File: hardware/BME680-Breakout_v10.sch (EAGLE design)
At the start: 23 parts, among them IC1 BME680, IC2 LDO-TS9011-3V3, J1 JUMPER2-0603, T1 BSS138PS, T2 BSS138PS, X1 PASSER-07, X2 PASSER-07

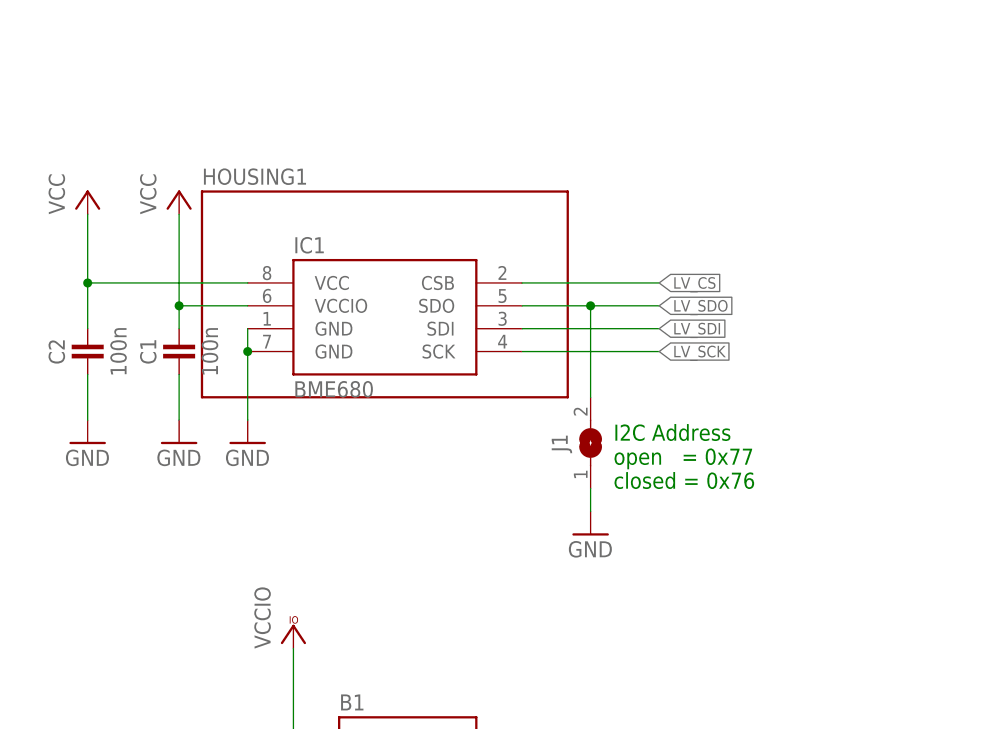
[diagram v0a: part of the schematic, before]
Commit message: updated layout and schematic
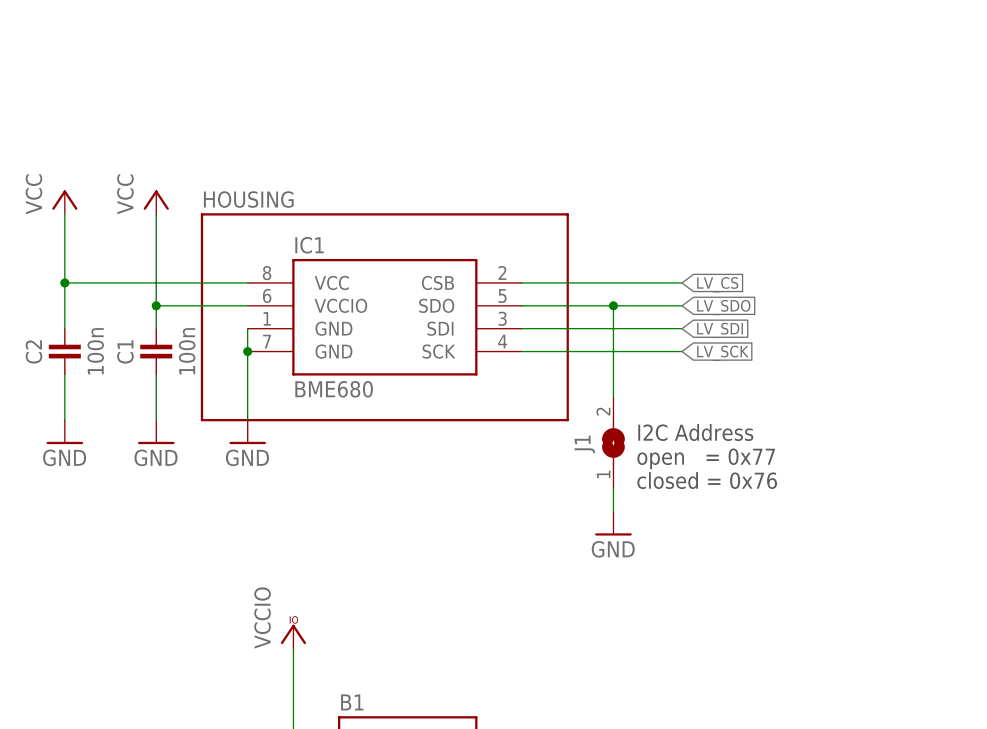
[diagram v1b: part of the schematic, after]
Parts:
- removed HOUSING1: SF2, we-sensor:SF2
- added HOUSING: SF2, we-sensor:SF2
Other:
- moved on the sheet: C1, C2, J1
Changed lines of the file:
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@@
 <setting verticaltext="up"/>
 </settings>
-<grid distance="0.1" unitdist="inch" unit="inch" style="lines" multiple="1" display="no" altdistance="0.01" altunitdist="inch" altunit="inch"/>
+<grid distance="0.05" unitdist="inch" unit="inch" style="lines" multiple="1" display="yes" altdistance="0.025" altunitdist="inch" altunit="inch"/>
 <layers>
 <layer number="1" name="Top" color="4" fill="1" visible="no" active="no"/>
@@
 <part name="J1" library="we-rcl" deviceset="JUMPER2" device="-0603"/>
 <part name="GND8" library="supply1" deviceset="GND" device=""/>
-<part name="HOUSING1" library="we-sensor" deviceset="SF2" device=""/>
+<part name="HOUSING" library="we-sensor" deviceset="SF2" device=""/>
 <part name="IC1" library="we-sensor" deviceset="BME680" device=""/>
 </parts>
@@
 <sheet>
 <plain>
-<text x="109.22" y="119.38" size="1.778" layer="91">I2C Address
+<text x="111.76" y="119.38" size="1.778" layer="97">I2C Address
 open   = 0x77
 closed = 0x76</text>
@@
 <instances>
 <instance part="B1" gate="BOARD" x="86.36" y="83.82"/>
-<instance part="GND1" gate="1" x="60.96" y="124.46"/>
-<instance part="P+1" gate="VCC" x="50.8" y="152.4"/>
-<instance part="C1" gate="C" x="60.96" y="134.62" rot="R90"/>
+<instance part="GND1" gate="1" x="58.42" y="124.46"/>
+<instance part="P+1" gate="VCC" x="48.26" y="152.4"/>
+<instance part="C1" gate="C" x="58.42" y="134.62" rot="R90"/>
 <instance part="R1" gate="R" x="191.77" y="154.94" rot="R90"/>
 <instance part="IC2" gate="A" x="86.36" y="43.18"/>
@@
 <attribute name="VALUE" x="201.93" y="33.02" size="1.778" layer="96"/>
 </instance>
-<instance part="P+2" gate="VCC" x="60.96" y="152.4"/>
-<instance part="C2" gate="C" x="50.8" y="134.62" rot="R90"/>
+<instance part="P+2" gate="VCC" x="58.42" y="152.4"/>
+<instance part="C2" gate="C" x="48.26" y="134.62" rot="R90"/>
 <instance part="GND2" gate="1" x="68.58" y="124.46"/>
-<instance part="GND3" gate="1" x="50.8" y="124.46"/>
+<instance part="GND3" gate="1" x="48.26" y="124.46"/>
 <instance part="R2" gate="R" x="217.17" y="154.94" rot="R90"/>
 <instance part="R3" gate="R" x="191.77" y="119.38" rot="R90"/>
@@
 <instance part="LOGO1" gate="L" x="207.01" y="7.62"/>
 <instance part="LOGO2" gate="L" x="194.31" y="7.62"/>
-<instance part="J1" gate="J" x="106.68" y="124.46" rot="R90"/>
-<instance part="GND8" gate="1" x="106.68" y="114.3"/>
-<instance part="HOUSING1" gate="G$1" x="83.82" y="139.7"/>
-<instance part="IC1" gate="G$1" x="83.82" y="137.16"/>
+<instance part="J1" gate="J" x="109.22" y="124.46" rot="R90"/>
+<instance part="GND8" gate="1" x="109.22" y="114.3"/>
+<instance part="HOUSING" gate="G$1" x="83.82" y="137.16"/>
+<instance part="IC1" gate="IC" x="83.82" y="137.16"/>
 </instances>
 <busses>
@@
 <segment>
 <pinref part="P+1" gate="VCC" pin="VCC"/>
-<wire x1="68.58" y1="142.24" x2="50.8" y2="142.24" width="0.1524" layer="91"/>
-<wire x1="50.8" y1="142.24" x2="50.8" y2="149.86" width="0.1524" layer="91"/>
+<wire x1="68.58" y1="142.24" x2="48.26" y2="142.24" width="0.1524" layer="91"/>
+<wire x1="48.26" y1="142.24" x2="48.26" y2="149.86" width="0.1524" layer="91"/>
 <pinref part="C2" gate="C" pin="2"/>
-<wire x1="50.8" y1="137.16" x2="50.8" y2="142.24" width="0.1524" layer="91"/>
-<junction x="50.8" y="142.24"/>
-<pinref part="IC1" gate="G$1" pin="VCC"/>
+<wire x1="48.26" y1="137.16" x2="48.26" y2="142.24" width="0.1524" layer="91"/>
+<junction x="48.26" y="142.24"/>
+<pinref part="IC1" gate="IC" pin="VCC"/>
 </segment>
 <segment>
 <pinref part="P+2" gate="VCC" pin="VCC"/>
-<wire x1="68.58" y1="139.7" x2="60.96" y2="139.7" width="0.1524" layer="91"/>
-<wire x1="60.96" y1="139.7" x2="60.96" y2="149.86" width="0.1524" layer="91"/>
+<wire x1="68.58" y1="139.7" x2="58.42" y2="139.7" width="0.1524" layer="91"/>
+<wire x1="58.42" y1="139.7" x2="58.42" y2="149.86" width="0.1524" layer="91"/>
 <pinref part="C1" gate="C" pin="2"/>
-<wire x1="60.96" y1="137.16" x2="60.96" y2="139.7" width="0.1524" layer="91"/>
-<junction x="60.96" y="139.7"/>
-<pinref part="IC1" gate="G$1" pin="VCCIO"/>
+<wire x1="58.42" y1="137.16" x2="58.42" y2="139.7" width="0.1524" layer="91"/>
+<junction x="58.42" y="139.7"/>
+<pinref part="IC1" gate="IC" pin="VCCIO"/>
 </segment>
 <segment>
@@
 <wire x1="68.58" y1="134.62" x2="68.58" y2="127" width="0.1524" layer="91"/>
 <junction x="68.58" y="134.62"/>
-<pinref part="IC1" gate="G$1" pin="GND@1"/>
-<pinref part="IC1" gate="G$1" pin="GND@2"/>
+<pinref part="IC1" gate="IC" pin="GND@1"/>
+<pinref part="IC1" gate="IC" pin="GND@2"/>
 </segment>
 <segment>
 <pinref part="GND3" gate="1" pin="GND"/>
 <pinref part="C2" gate="C" pin="1"/>
-<wire x1="50.8" y1="127" x2="50.8" y2="132.08" width="0.1524" layer="91"/>
+<wire x1="48.26" y1="127" x2="48.26" y2="132.08" width="0.1524" layer="91"/>
 </segment>
 <segment>
 <pinref part="C1" gate="C" pin="1"/>
 <pinref part="GND1" gate="1" pin="GND"/>
-<wire x1="60.96" y1="132.08" x2="60.96" y2="127" width="0.1524" layer="91"/>
+<wire x1="58.42" y1="132.08" x2="58.42" y2="127" width="0.1524" layer="91"/>
 </segment>
 <segment>
@@
 <pinref part="GND8" gate="1" pin="GND"/>
 <pinref part="J1" gate="J" pin="1"/>
-<wire x1="106.68" y1="116.84" x2="106.68" y2="119.38" width="0.1524" layer="91"/>
+<wire x1="109.22" y1="116.84" x2="109.22" y2="119.38" width="0.1524" layer="91"/>
 </segment>
 </net>
 <net name="LV_SDO" class="0">
 <segment>
-<wire x1="99.06" y1="139.7" x2="106.68" y2="139.7" width="0.1524" layer="91"/>
-<label x="114.3" y="139.7" size="1.27" layer="95" xref="yes"/>
+<wire x1="99.06" y1="139.7" x2="109.22" y2="139.7" width="0.1524" layer="91"/>
+<label x="116.84" y="139.7" size="1.27" layer="95" xref="yes"/>
 <pinref part="J1" gate="J" pin="2"/>
-<wire x1="106.68" y1="139.7" x2="114.3" y2="139.7" width="0.1524" layer="91"/>
-<wire x1="106.68" y1="129.54" x2="106.68" y2="139.7" width="0.1524" layer="91"/>
-<junction x="106.68" y="139.7"/>
-<pinref part="IC1" gate="G$1" pin="SDO"/>
+<wire x1="109.22" y1="139.7" x2="116.84" y2="139.7" width="0.1524" layer="91"/>
+<wire x1="109.22" y1="129.54" x2="109.22" y2="139.7" width="0.1524" layer="91"/>
+<junction x="109.22" y="139.7"/>
+<pinref part="IC1" gate="IC" pin="SDO"/>
 </segment>
 <segment>
@@
 <net name="LV_CS" class="0">
 <segment>
-<wire x1="99.06" y1="142.24" x2="114.3" y2="142.24" width="0.1524" layer="91"/>
-<label x="114.3" y="142.24" size="1.27" layer="95" xref="yes"/>
-<pinref part="IC1" gate="G$1" pin="CSB"/>
+<wire x1="99.06" y1="142.24" x2="116.84" y2="142.24" width="0.1524" layer="91"/>
+<label x="116.84" y="142.24" size="1.27" layer="95" xref="yes"/>
+<pinref part="IC1" gate="IC" pin="CSB"/>
 </segment>
 <segment>
@@
 <net name="LV_SDI" class="0">
 <segment>
-<wire x1="99.06" y1="137.16" x2="114.3" y2="137.16" width="0.1524" layer="91"/>
-<label x="114.3" y="137.16" size="1.27" layer="95" xref="yes"/>
-<pinref part="IC1" gate="G$1" pin="SDI"/>
+<wire x1="99.06" y1="137.16" x2="116.84" y2="137.16" width="0.1524" layer="91"/>
+<label x="116.84" y="137.16" size="1.27" layer="95" xref="yes"/>
+<pinref part="IC1" gate="IC" pin="SDI"/>
 </segment>
 <segment>
@@
 <net name="LV_SCK" class="0">
 <segment>
-<wire x1="99.06" y1="134.62" x2="114.3" y2="134.62" width="0.1524" layer="91"/>
-<label x="114.3" y="134.62" size="1.27" layer="95" xref="yes"/>
-<pinref part="IC1" gate="G$1" pin="SCK"/>
-</segment>
-<segment>
+<wire x1="99.06" y1="134.62" x2="116.84" y2="134.62" width="0.1524" layer="91"/>
+<label x="116.84" y="134.62" size="1.27" layer="95" xref="yes"/>
+<pinref part="IC1" gate="IC" pin="SCK"/>
+</segment>
+<segment>
